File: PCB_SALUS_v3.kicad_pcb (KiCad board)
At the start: 2 copper layers, 100 x 100 mm, 103 parts, among them J1 Debug_U0, J10 RELES_2, J11 Throttle, J12 I2C_EXT1, J13 I2C_EXT2, J14 S_HALL, J15 RF_PPM, J16 USB_NATIVO, J17 SERVO2, J18 SERVO1, J19 +7V_IN, J2 S_GIRO, J20 3V_IN, J3 USB_UART0, J4 Uart1, J5 5V_IN, J6 IBT_2, J7 FC1, J8 FC2, J9 RELES_1, Q3 SS8050, Q4 SS8050, U3 CP2102N-A02-GQFN24, U4 BMI088, U5 74HC595, U6 ULN2003A, U7 LM358, U8 ESP32-S3-WROOM-1, U9 AP63203WU

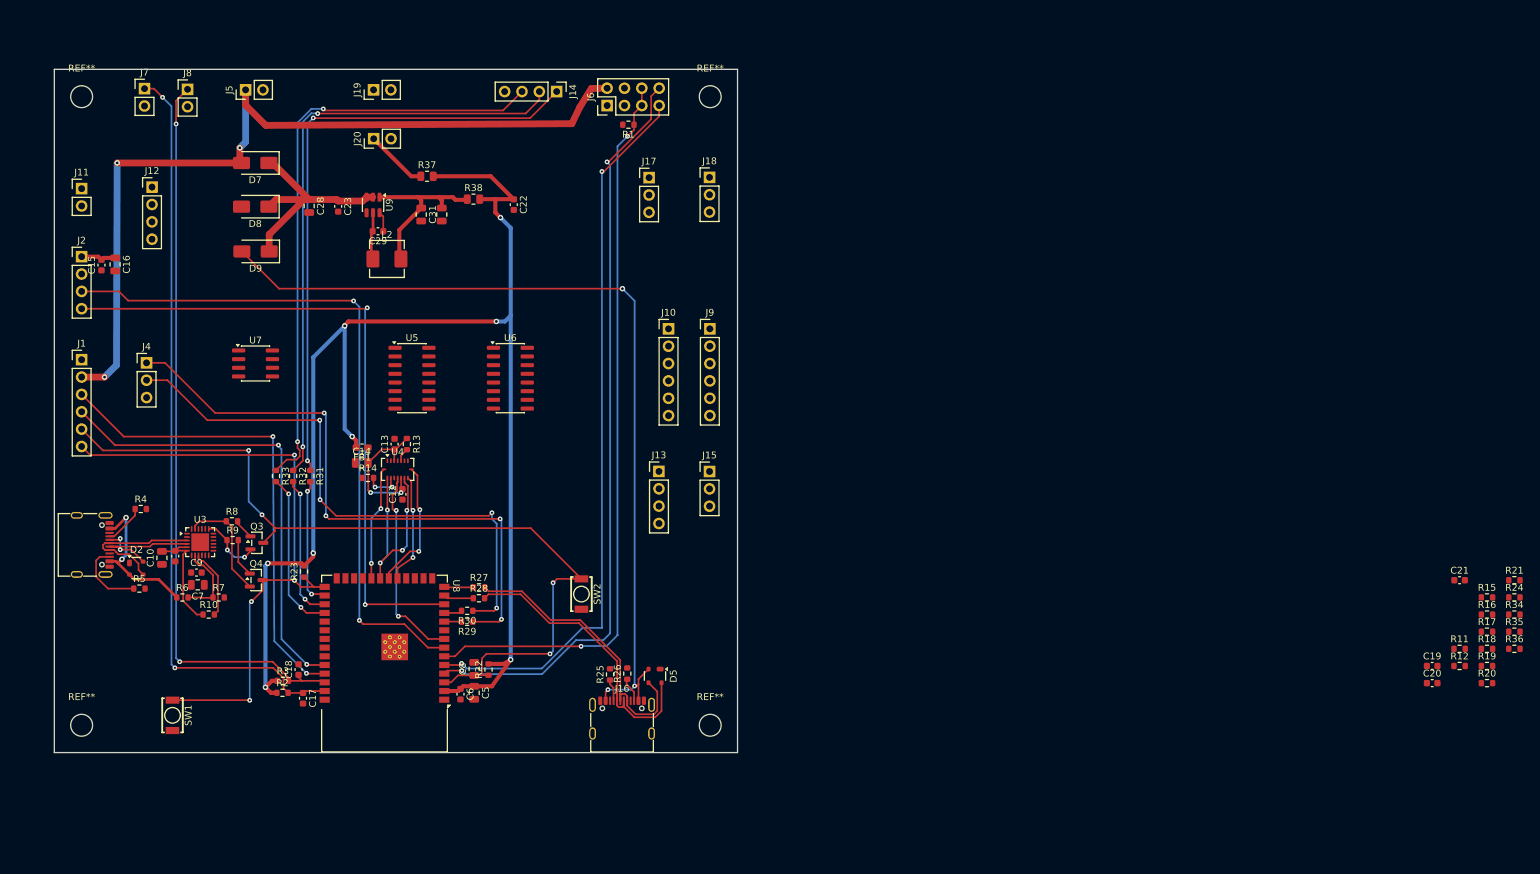
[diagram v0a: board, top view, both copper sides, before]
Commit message: routeo terminado v1
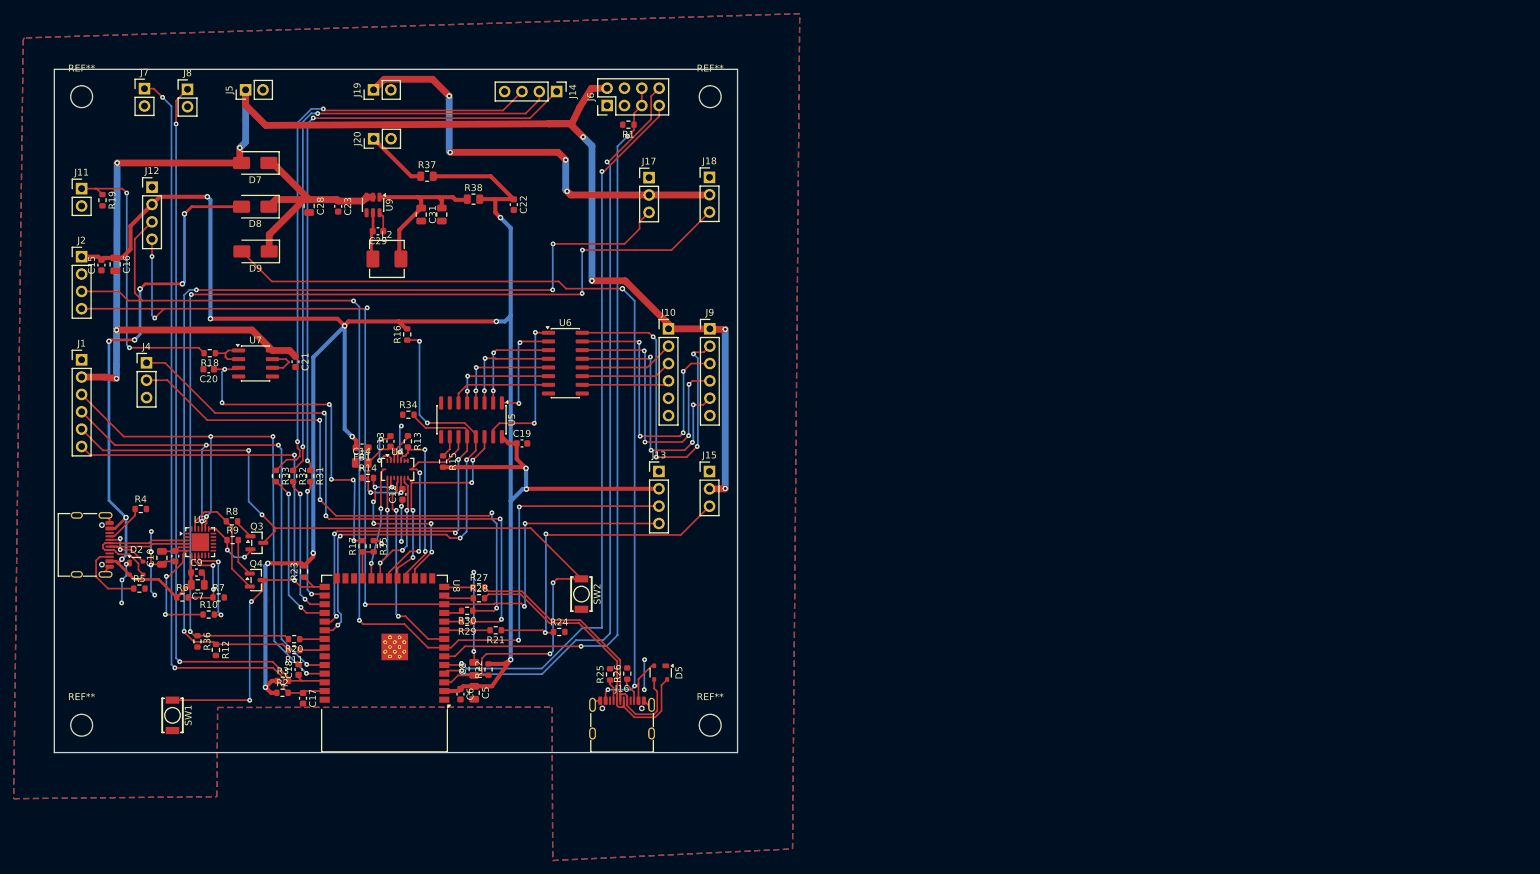
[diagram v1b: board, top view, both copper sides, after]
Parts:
- moved R19 213.8 mm to (57.0, 69.2), turned to -90 degrees
- moved R36 192.8 mm to (71.0, 133.7), turned to -90 degrees
- moved R18 191.9 mm to (72.8, 91.5), turned to 180 degrees
- moved C20 184.9 mm to (72.6, 93.9), turned to 180 degrees
- moved R12 182.0 mm to (73.7, 135.0), turned to -90 degrees
- moved R20 174.7 mm to (85.1, 133.4), turned to 180 degrees
- moved C21 173.4 mm to (85.3, 92.8), turned to -90 degrees
- moved R11 170.6 mm to (85.1, 135.0), turned to 180 degrees
- moved R35 167.4 mm to (96.8, 119.8), turned to -90 degrees
- moved R17 165.1 mm to (95.1, 119.8), turned to 90 degrees
- moved R34 164.5 mm to (101.8, 100.5)
- moved R16 163.3 mm to (101.7, 88.8), turned to 90 degrees
- moved R15 154.1 mm to (106.9, 107.4), turned to -90 degrees
- moved R21 149.3 mm to (114.6, 132.1), turned to 180 degrees
- moved R24 139.9 mm to (123.9, 132.3)
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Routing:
- net Net-(J18-Pin_3): track 0.00 -> 148.8 mm, vias 0 -> 4
- net Net-(J17-Pin_3): track 0.00 -> 143.3 mm, vias 0 -> 4
- net +5V: track 124.2 -> 229.2 mm, vias 3 -> 8
- net +3.3V: track 216.1 -> 319.7 mm, vias 8 -> 12
- net RELAY_OE: track 0.00 -> 71.9 mm, vias 0 -> 6
- net USB_VBUS: track 22.3 -> 93.6 mm, vias 2 -> 7
- net GND: track 0.00 -> 65.5 mm, vias 0 -> 18
- net I2C_SDA: track 101.6 -> 166.0 mm, vias 2 -> 4
- net +7V: track 0.00 -> 64.2 mm, vias 0 -> 4
- net I2C_SCL: track 97.0 -> 154.4 mm, vias 2 -> 6
- net RELAY_LATCH: track 0.00 -> 56.8 mm, vias 0 -> 4
- net Net-(J9-Pin_2): track 0.00 -> 51.8 mm, vias 0 -> 4
- net Net-(U7A-+): track 0.00 -> 49.1 mm, vias 0 -> 6
- net Net-(J15-Pin_3): track 0.00 -> 48.1 mm, vias 0 -> 2
- net /SENSORES/THROTTLE_OUT: track 0.00 -> 42.4 mm, vias 0 -> 2
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- added copper zone on B.Cu, net GND
- added copper zone on F.Cu, net GND
